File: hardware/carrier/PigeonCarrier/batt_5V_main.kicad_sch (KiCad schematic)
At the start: 1 part, among them U1 LM61495RPHR

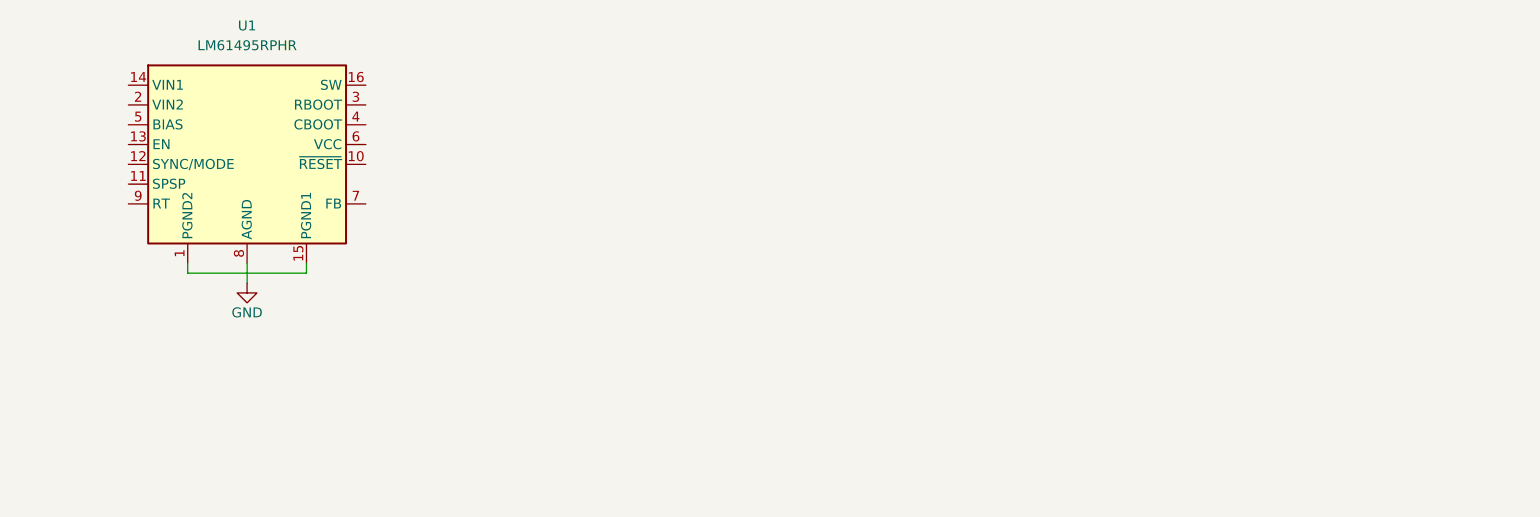
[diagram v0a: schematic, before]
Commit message: carrier progress
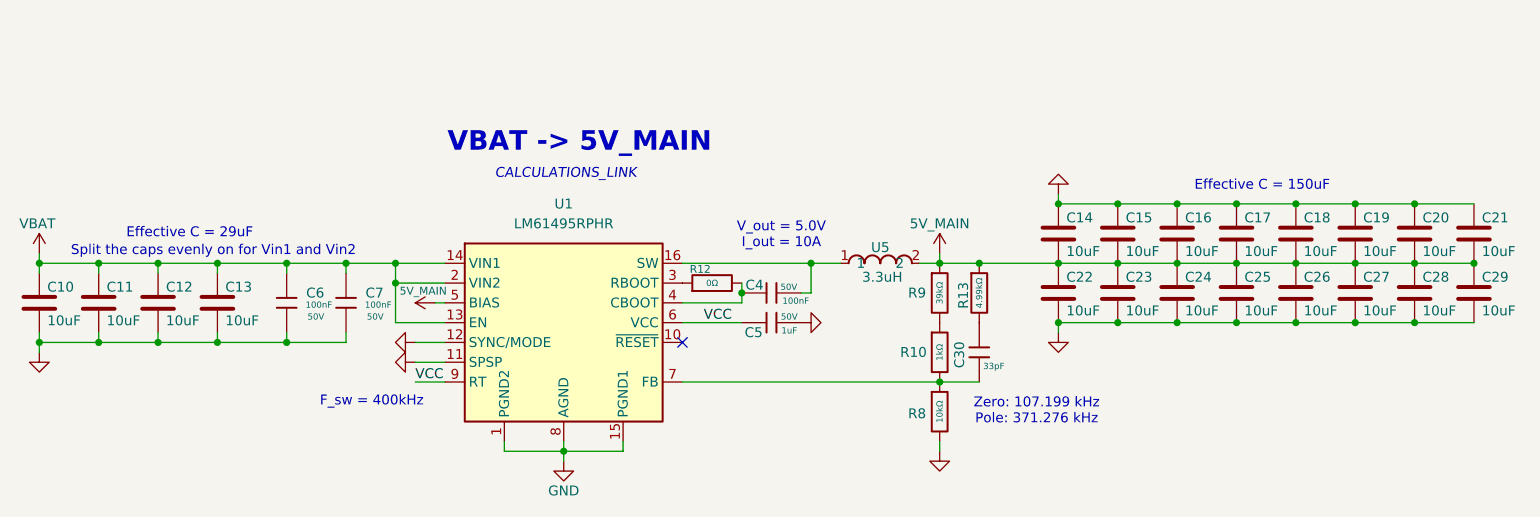
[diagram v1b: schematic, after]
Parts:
- added C10, C11, C12, C13, C14, C15, C16, C17, C18, C19, C20, C21, C22, C23, C24, C25, C26, C27, C28, C29: 10uF, Capacitor_SMD:C_1210_3225Metric, symbol Device:C
- added C30: 33pF, PCM_JLCPCB:C_0402, symbol PCM_JLCPCB-Capacitors:0402,33pF
- added C4, C6, C7: 100nF, PCM_JLCPCB:C_0402, symbol PCM_JLCPCB-Capacitors:0402,100nF,(2)
- added C5: 1uF, PCM_JLCPCB:C_0603, symbol PCM_JLCPCB-Capacitors:0603,1uF
- added R10: 1kΩ, PCM_JLCPCB:R_0402, symbol PCM_JLCPCB-Resistors:0402,1kΩ
- added R12: 0Ω, PCM_JLCPCB:R_0402, symbol PCM_JLCPCB-Resistors:0402,0Ω
- added R13: 4.99kΩ, PCM_JLCPCB:R_0603, symbol PCM_JLCPCB-Resistors:0603,4.99kΩ
- added R8: 10kΩ, PCM_JLCPCB:R_0402, symbol PCM_JLCPCB-Resistors:0402,10kΩ
- added R9: 39kΩ, PCM_JLCPCB:R_0402, symbol PCM_JLCPCB-Resistors:0402,39kΩ
- added U5: 3.3uH, JLCImport_Auto:CYA1265-3_3UH, symbol JLCImport_Auto:CYA1265-3_3UH
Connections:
- net GND: now also U1.1 (PGND2), U1.11 (SPSP), U1.12 (SYNC/MODE), U1.15 (PGND1), C10.2, C11.2, C12.2, C13.2, C14.1, C15.1, C16.1, C17.1, C18.1, C19.1, C20.1, C21.1, C22.2, C23.2, C24.2, C25.2, C26.2, C27.2, C28.2, C29.2, C5.2, C6.1, C7.1, R8.2
- net VBAT: now reaches U1.13 (EN)
- net VBAT: now also U1.14 (VIN1), U1.2 (VIN2), C10.1, C11.1, C12.1, C13.1, C6.2, C7.2
- net at U1.16 (SW): now also C4.2, U5.1
- net at U1.3 (RBOOT): now also R12.1
- net at U1.4 (CBOOT): now also C4.1, R12.2
- net 5V_MAIN: now reaches U1.5 (BIAS)
- net 5V_MAIN: now also C14.2, C15.2, C16.2, C17.2, C18.2, C19.2, C20.2, C21.2, C22.1, C23.1, C24.1, C25.1, C26.1, C27.1, C28.1, C29.1, R13.1, R9.1, U5.2
- net VCC: now reaches U1.6 (VCC)
- net VCC: now also U1.9 (RT), C5.1
- net at U1.7 (FB): now also C30.2, R10.2, R8.1
- new net: C30.1, R13.2
- new net: R10.1, R9.2
- no-connect marks 0 -> 1
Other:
- note added: "CALCULATIONS_LINK"
- note added: "Effective C = 150uF"
- note added: "Effective C = 29uF"
- note added: "F_sw = 400kHz"
- note added: "I_out = 10A"
- note added: "Split the caps evenly on for Vin1 and Vin2"
- note added: "VBAT -> 5V_MAIN"
- note added: "V_out = 5.0V"
- note added: "Zero: 107.199 kHz Pole: 371.276 kHz"
- moved on the sheet: U1
